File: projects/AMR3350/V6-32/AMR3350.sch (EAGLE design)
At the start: 243 parts, among them IC1 LDO-TS1117CW-3V3, IC10 TMC21X0-LA, IC11 74LS32D, IC2 ATSAM4S8C, IC3 SI87XXIS, IC4 74HC125, IC5 74S08D, IC6 TMC21X0-LA, IC7 TMC21X0-LA, IC8 TMC21X0-LA, IC9 TMC21X0-LA, J1 MOLEX-105162-001, J2 MSTBV4, Q1 NX138BKS, Q2 NX138BKS, Q3 BUK9Y53-100B, Q4 BUK9Y53-100B, U1 A4403, X1 USB-B_TH, X2 12MHz, X3 KK-254-2, X4 KK-254-4, X5 KK-254-4, X6 KK-254-4, X7 KK-254-4, X8 KK-254-4, X9 KK-254-4

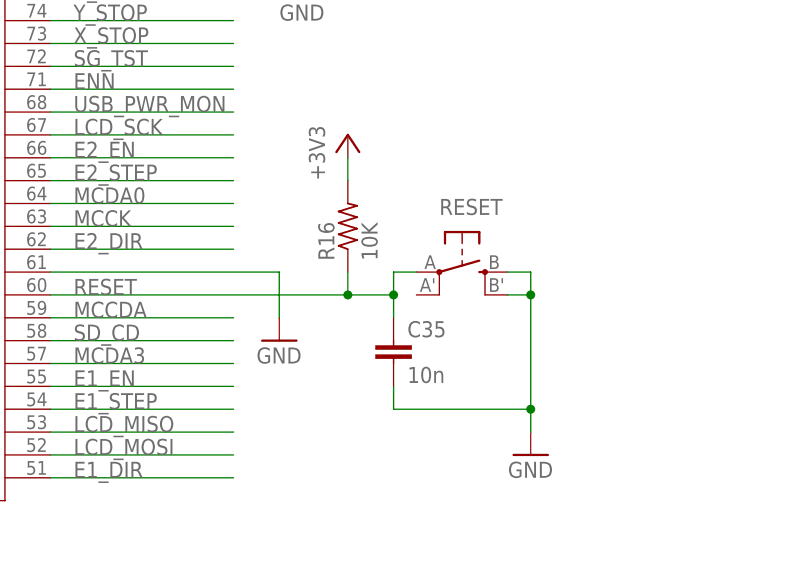
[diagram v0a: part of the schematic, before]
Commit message: Done***
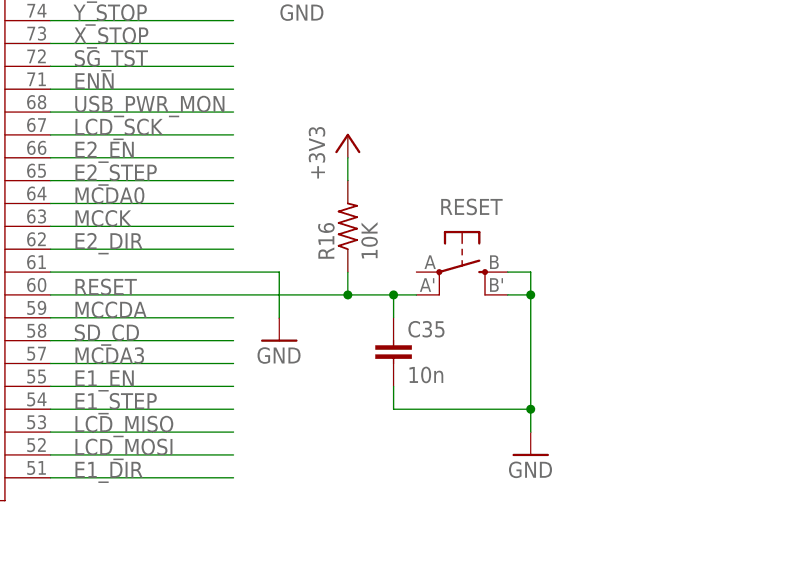
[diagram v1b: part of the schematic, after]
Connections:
- net RESET: now also RESET.P1; no longer RESET.P
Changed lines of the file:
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@@
 <wire x1="332.74" y1="-33.02" x2="332.74" y2="-30.48" width="0.1524" layer="91"/>
 <junction x="332.74" y="-30.48"/>
-<pinref part="RESET" gate="G$1" pin="P"/>
-<wire x1="332.74" y1="-30.48" x2="332.74" y2="-27.94" width="0.1524" layer="91"/>
-<wire x1="332.74" y1="-27.94" x2="335.28" y2="-27.94" width="0.1524" layer="91"/>
 <label x="297.18" y="-30.48" size="1.778" layer="95"/>
+<pinref part="RESET" gate="G$1" pin="P1"/>
+<wire x1="332.74" y1="-30.48" x2="335.28" y2="-30.48" width="0.1524" layer="91"/>
 </segment>
 </net>
